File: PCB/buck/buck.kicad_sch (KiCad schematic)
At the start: 12 parts, among them J1 UBat 38V, J2 Uout 5V, J3 Zündung, Q1 QM6006D, U1 LM2575-5.0BT

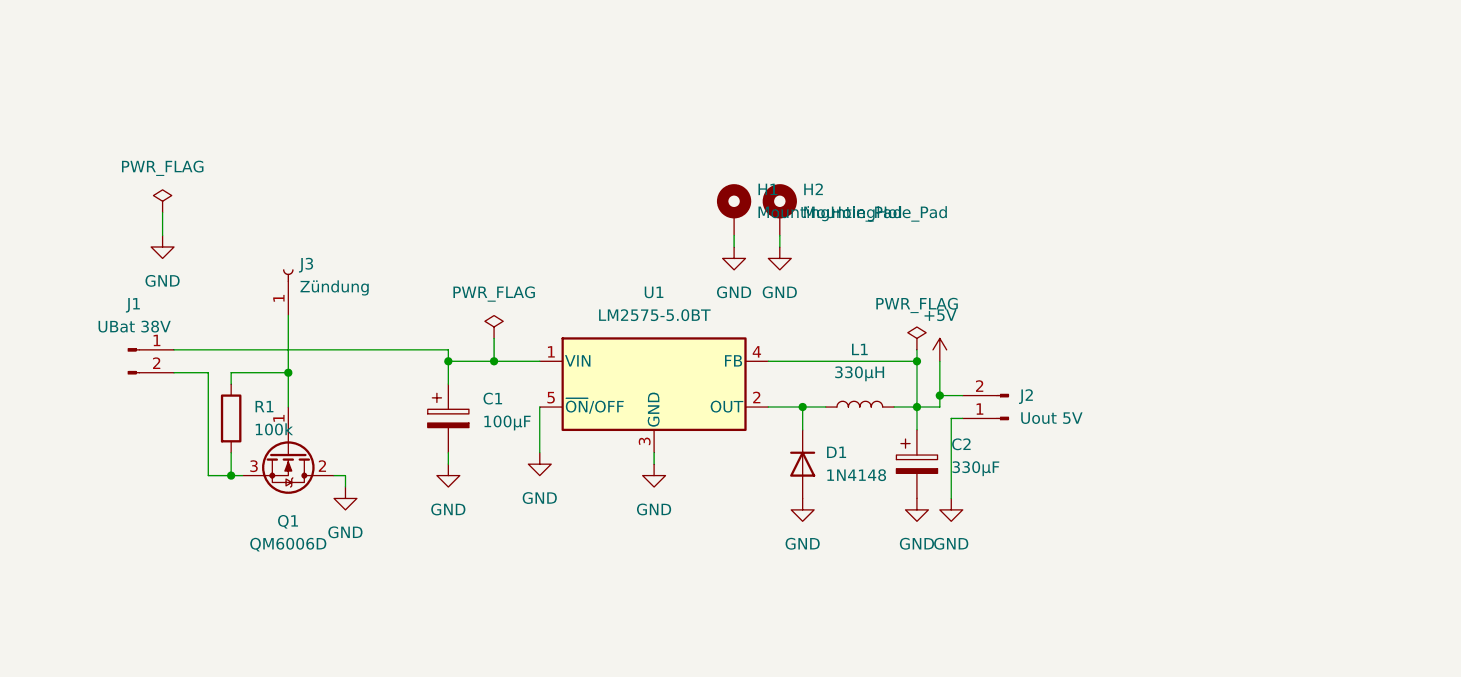
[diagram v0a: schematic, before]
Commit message: Release v1.0
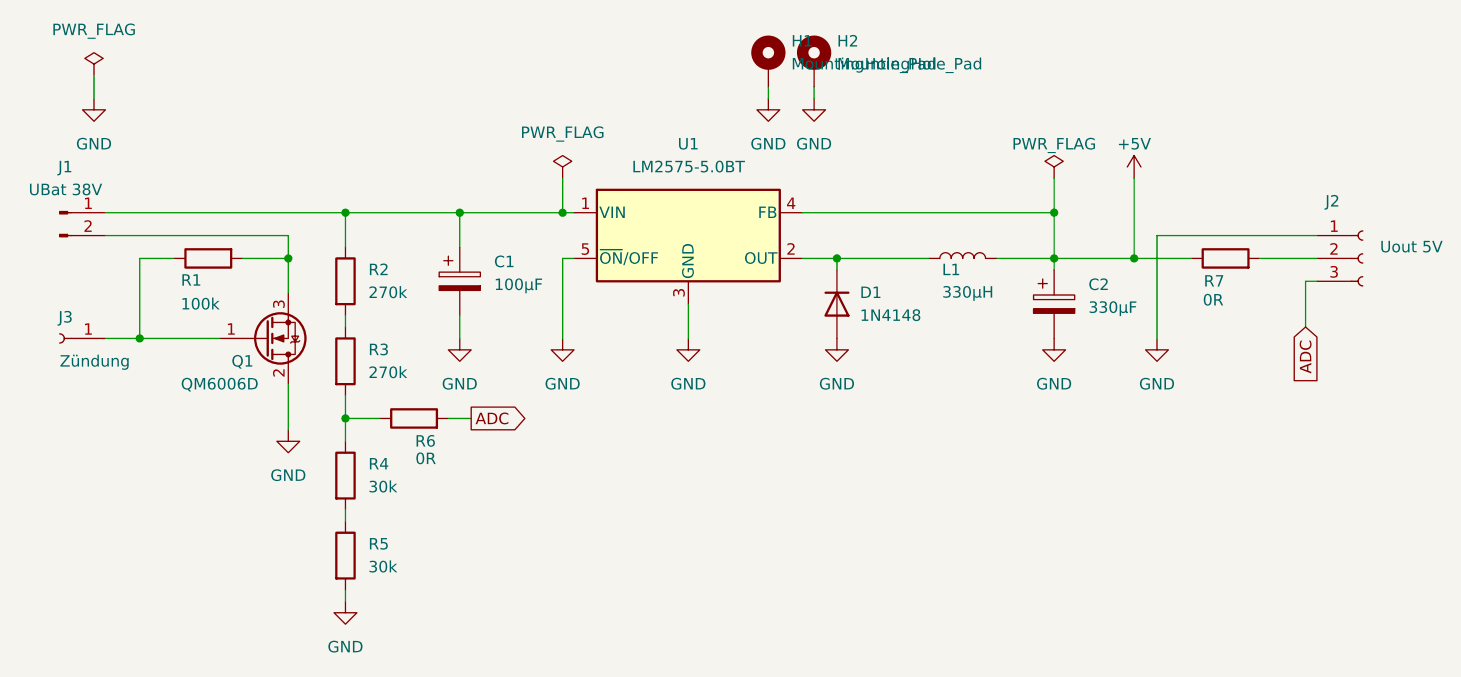
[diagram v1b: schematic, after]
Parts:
- added R2, R3: 270k, Resistor_SMD:R_0805_2012Metric, symbol Device:R
- added R4, R5: 30k, Resistor_SMD:R_0805_2012Metric, symbol Device:R
- added R6, R7: 0R, Resistor_SMD:R_0603_1608Metric, symbol Device:R
- J2: footprint Connector_PinSocket_2.54mm:PinSocket_1x02_P2.54mm_Horizontal -> Connector_PinSocket_2.54mm:PinSocket_1x03_P2.54mm_Horizontal; symbol Connector:Conn_01x02_Male -> Connector:Conn_01x03_Female
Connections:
- net +5V: now also R7.1; no longer J2.2 (Pin_2)
- net GND: now also R5.2
- net at C1.1, J1.1 (Pin_1), U1.1 (VIN): now also R2.1
- new net: R3.2, R4.1, R6.1
- new net: R2.2, R3.1
- new net: J2.2 (Pin_2), R7.2
- new net: R4.2, R5.1
- new net ADC: J2.3 (Pin_3), R6.2
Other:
- moved on the sheet: C1, C2, D1, H1, H2, J1, J3, L1, Q1, R1, U1
